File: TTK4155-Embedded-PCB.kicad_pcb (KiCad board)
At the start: 2 copper layers, 42 parts, among them J1 AVR-JTAG-10, J2 DB9_Female, J3 Conn_01x10_Male, J4 Conn_01x04_Male, J5 Screw_Terminal_01x02, J6 Screw_Terminal_01x02, SW1 SW_Push, U1 L7805, U2 ATmega162-16PU, U3 IDT7164S, U4 GAL16V8, U5 SN74ALS573CN, U6 MCP2515-18PDIP, U7 MCP2551-I-P, U8 MAX233, U9 ADC0844, Y1 4,9152MHz, Y2 16.0MHz

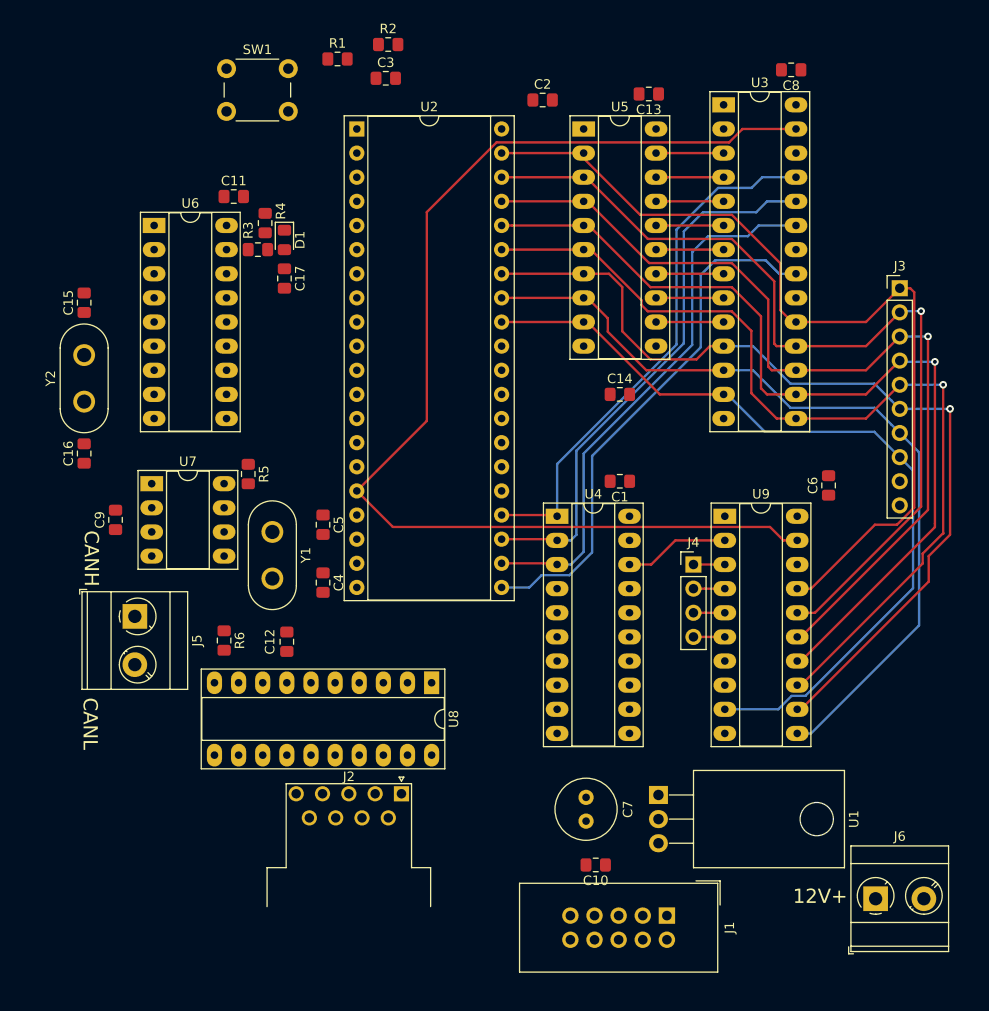
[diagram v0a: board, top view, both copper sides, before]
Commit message: Finished first revision of board
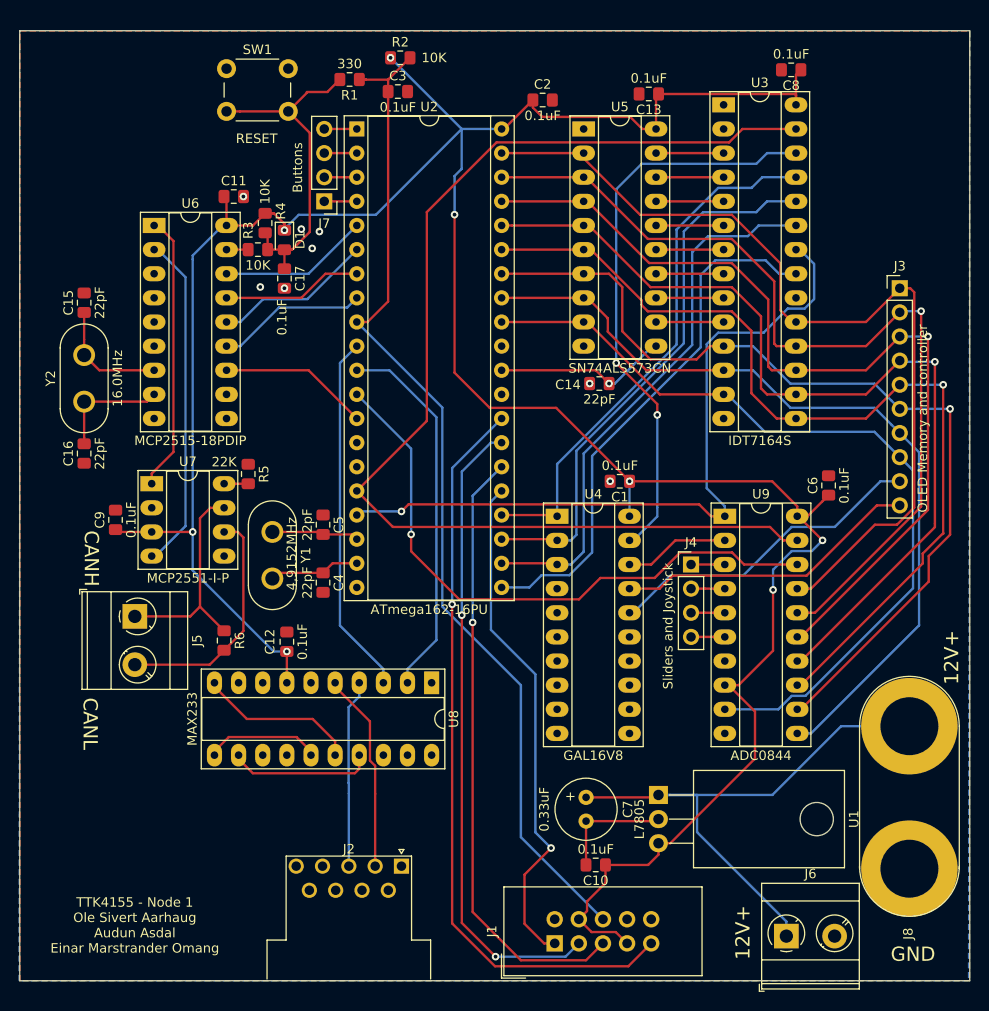
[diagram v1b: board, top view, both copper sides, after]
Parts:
- added J7: Conn_01x04_Male, Connector_PinHeader_2.54mm:PinHeader_1x04_P2.54mm_Vertical, F.Cu at (74.3, 49.8)
- added J8: BannanaJack, TTK4155-Embedded-PCB:Banana_Jack_2Pin_15mm_spacing, F.Cu at (135.9, 105.0)
- moved J1 12.2 mm to (98.6, 127.9), turned to 90 degrees
- moved J6 10.2 mm to (122.9, 127.1)
- moved J2 7.62 mm to (82.4, 119.8)
- moved R1 2.50 mm to (77.0, 37.0), turned to 180 degrees
- moved C14 2.44 mm to (103.3, 69.0)
- moved R2 1.89 mm to (82.3, 34.7)
- moved C3 1.89 mm to (82.0, 38.2)
- moved J4 0.25 mm to (112.9, 88.0)
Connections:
- J6 pad 1: Net-(J6-Pad1) -> +12V
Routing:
- net +5V: track 0.00 -> 299.8 mm, vias 0 -> 8
- net /~RESET: track 0.00 -> 107.4 mm
- net /TDI: track 0.00 -> 79.1 mm, vias 0 -> 1
- net /~OE: track 0.00 -> 78.1 mm, vias 0 -> 1
- net /TDO: track 0.00 -> 67.3 mm, vias 0 -> 2
- net /TMS: track 0.00 -> 64.7 mm, vias 0 -> 1
- net /INT0: track 0.00 -> 64.2 mm, vias 0 -> 1
- net /CS_RAM: track 0.00 -> 60.7 mm, vias 0 -> 2
- net +12V: track 0.00 -> 60.0 mm
- net /TCK: track 0.00 -> 53.8 mm, vias 0 -> 1
- net /TXD0: track 0.00 -> 39.6 mm
- net /RXD0: track 0.00 -> 38.1 mm
- net /~RESETCAN: track 0.00 -> 36.1 mm
- net /RXCAN: track 0.00 -> 35.6 mm
- net /OLED_DATA: track 0.00 -> 34.2 mm
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- added copper zone on B.Cu, net GND
- added copper zone on F.Cu, net GND
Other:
- board outline added: 100 x 100 mm
- board text added: "+"
- board text added: "Buttons"
- board text added: "GND"
- board text added: "OLED Memory and controller"
- board text added: "RESET"
- board text added: "Sliders and Joystick"
- board text added: "TTK4155 - Node 1 Ole Sivert Aarhaug Audun Asdal Einar Marstrander Omang"
